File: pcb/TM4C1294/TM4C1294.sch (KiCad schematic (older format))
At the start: 38 parts, among them J1 EK-TM4C1294, Q1 PN2222A, Q2 PN2222A, Q3 PN2222A, Q4 PN2222A, T1 Keypad4x4, U1 CA56-12CGKWA

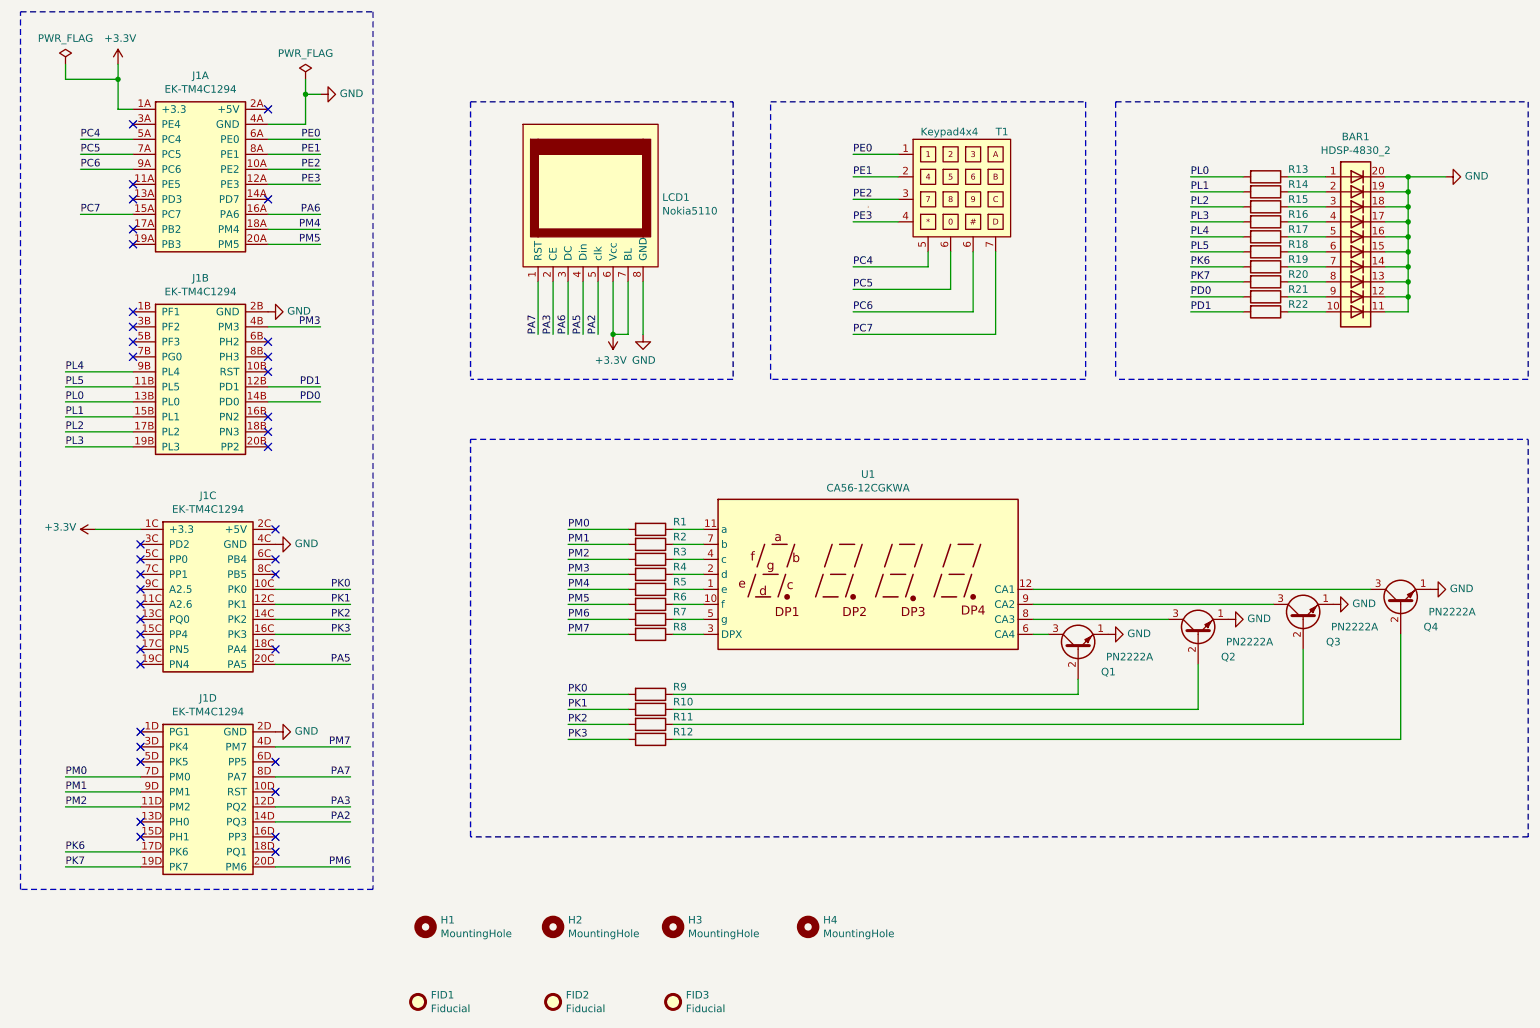
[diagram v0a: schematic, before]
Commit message: Version 1.0
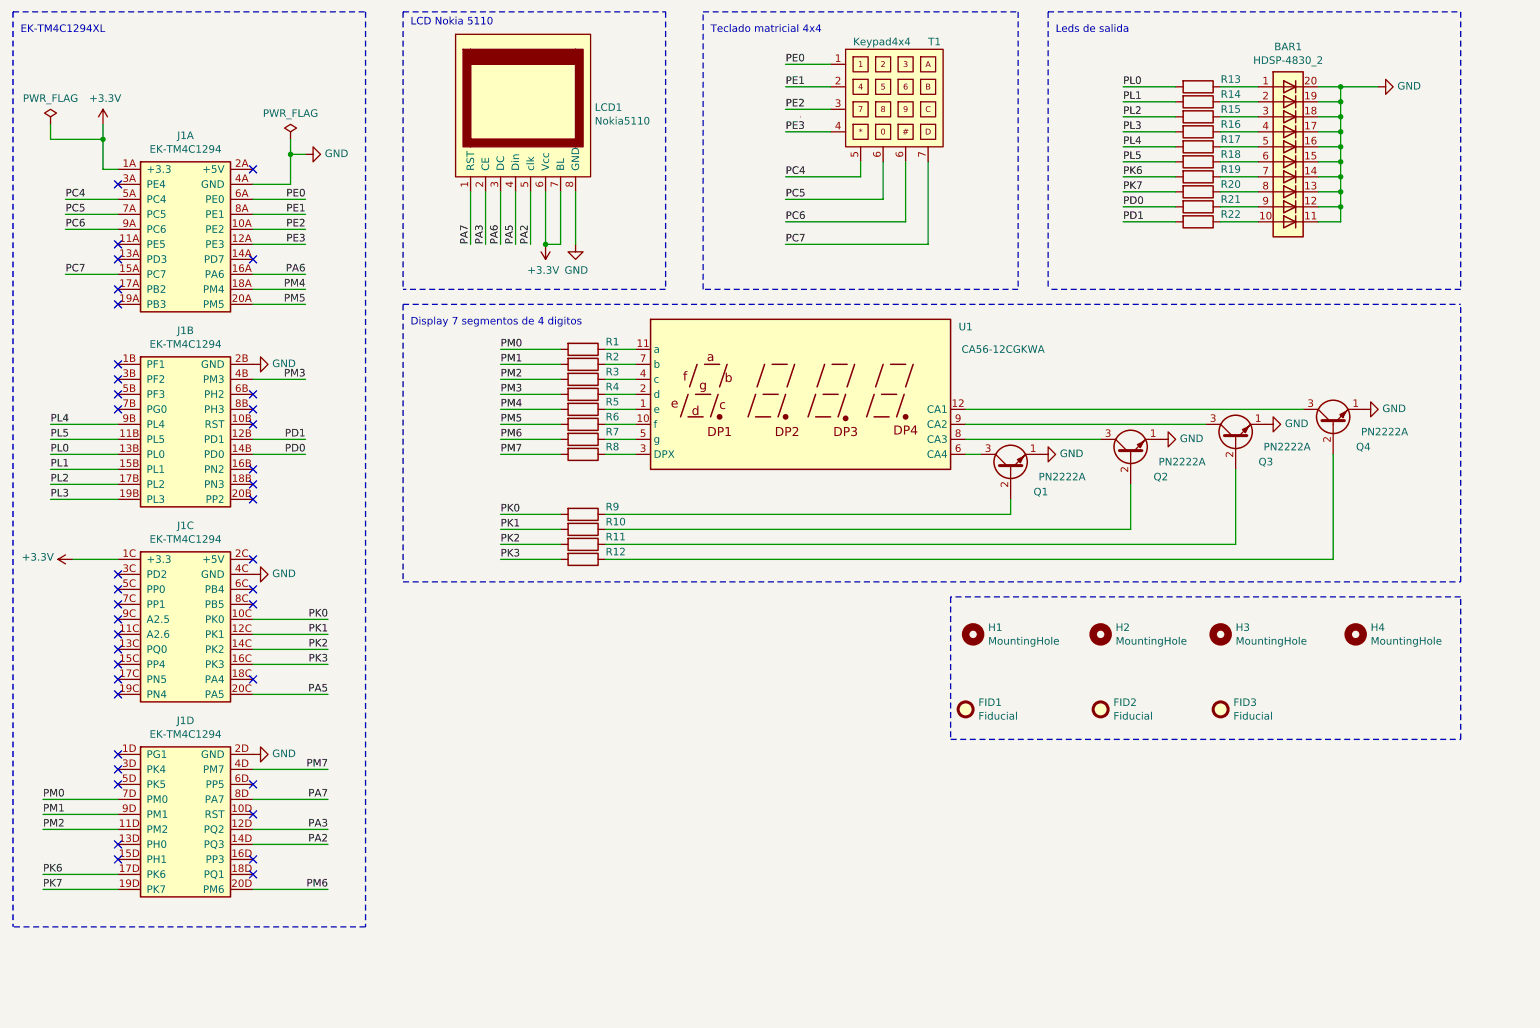
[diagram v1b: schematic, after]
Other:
- note added: "Display 7 segmentos de 4 digitos"
- note added: "EK-TM4C1294XL"
- note added: "LCD Nokia 5110\n"
- note added: "Leds de salida"
- note added: "Teclado matricial 4x4"
- moved on the sheet: BAR1, FID1, FID2, FID3, H1, H2, H3, H4, J1A, J1B, J1C, J1D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
